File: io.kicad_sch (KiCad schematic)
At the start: 20 parts, among them J3 USB_C_Receptacle_USB2.0, J4 Conn_01x06_Male, U3 USBLC6-2SC6

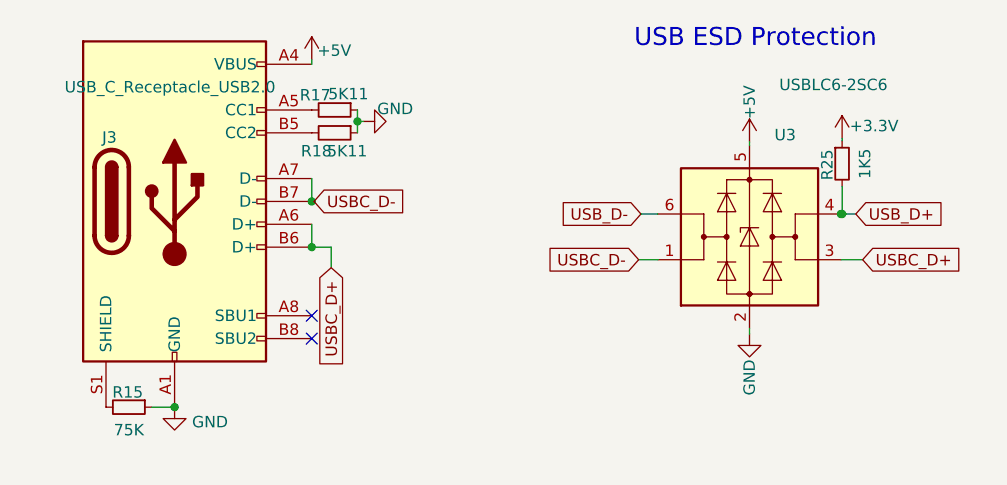
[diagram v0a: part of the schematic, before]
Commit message: kicad - 7
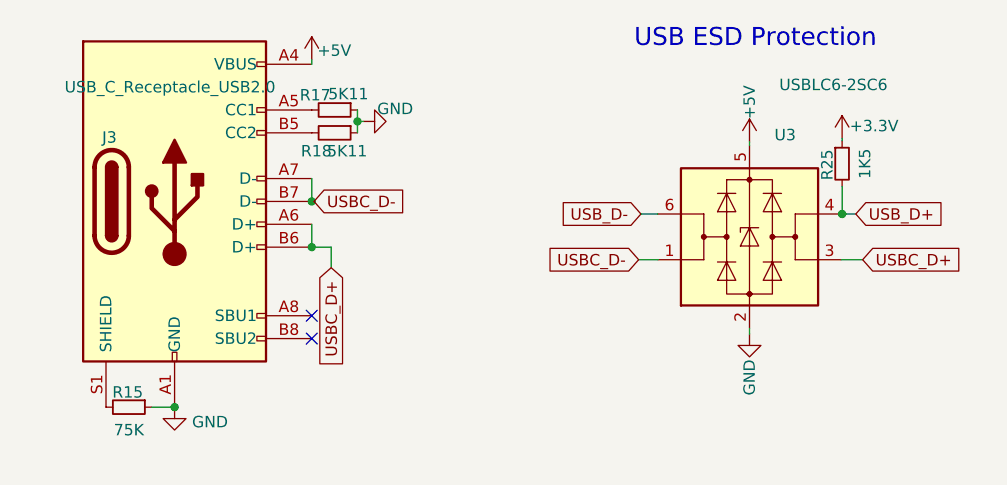
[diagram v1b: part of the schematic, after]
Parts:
- J4: footprint Connector_PinHeader_2.54mm:PinHeader_2x03_P2.54mm_Vertical -> easyeda2kicad:HDR-TH_6P-P2.54-H-M-R2-C3-S2.54
